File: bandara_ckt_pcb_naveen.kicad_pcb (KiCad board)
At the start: 2 copper layers, 98.8 x 78.6 mm, 54 parts, among them J1 Nanopore, U1 MCP4725xxx-xCH, U2 ADS1115IDGS, U3 AD820, U4 Dual Power Supply, U5 AD820, U6 AD820

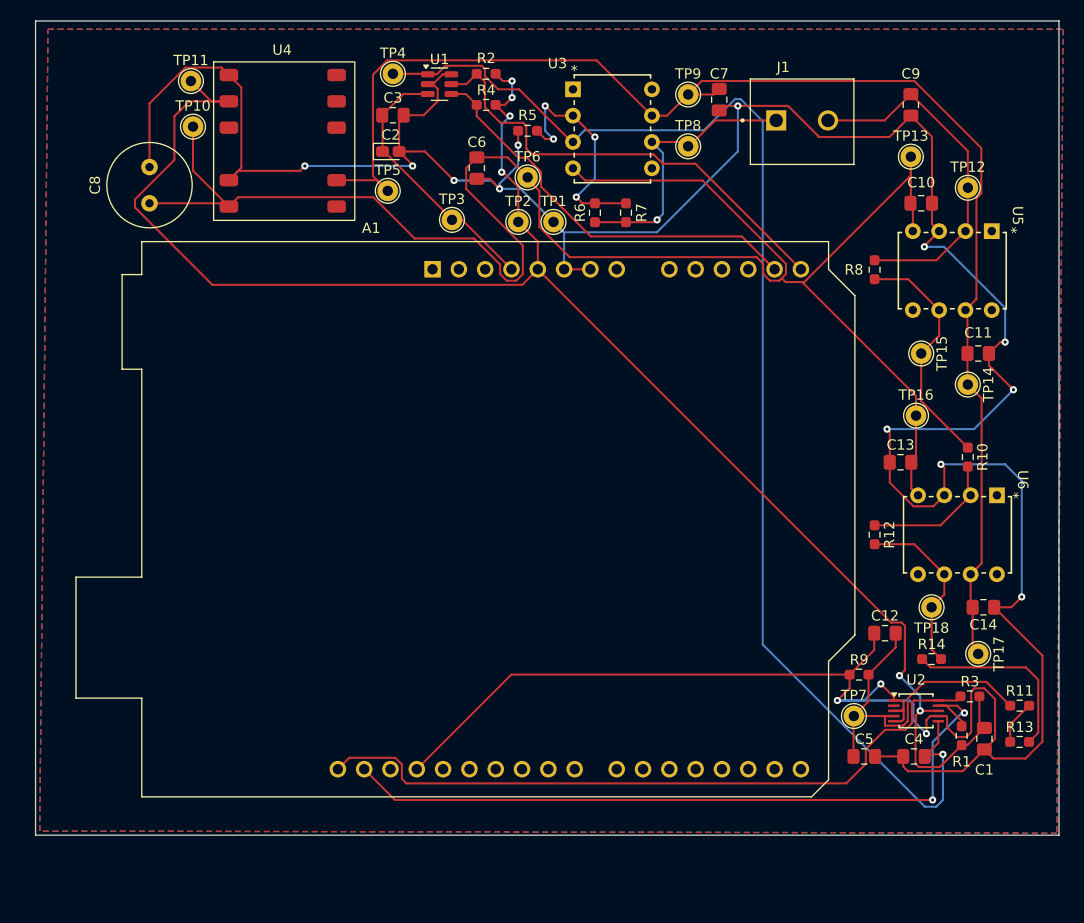
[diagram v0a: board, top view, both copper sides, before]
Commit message: Changes
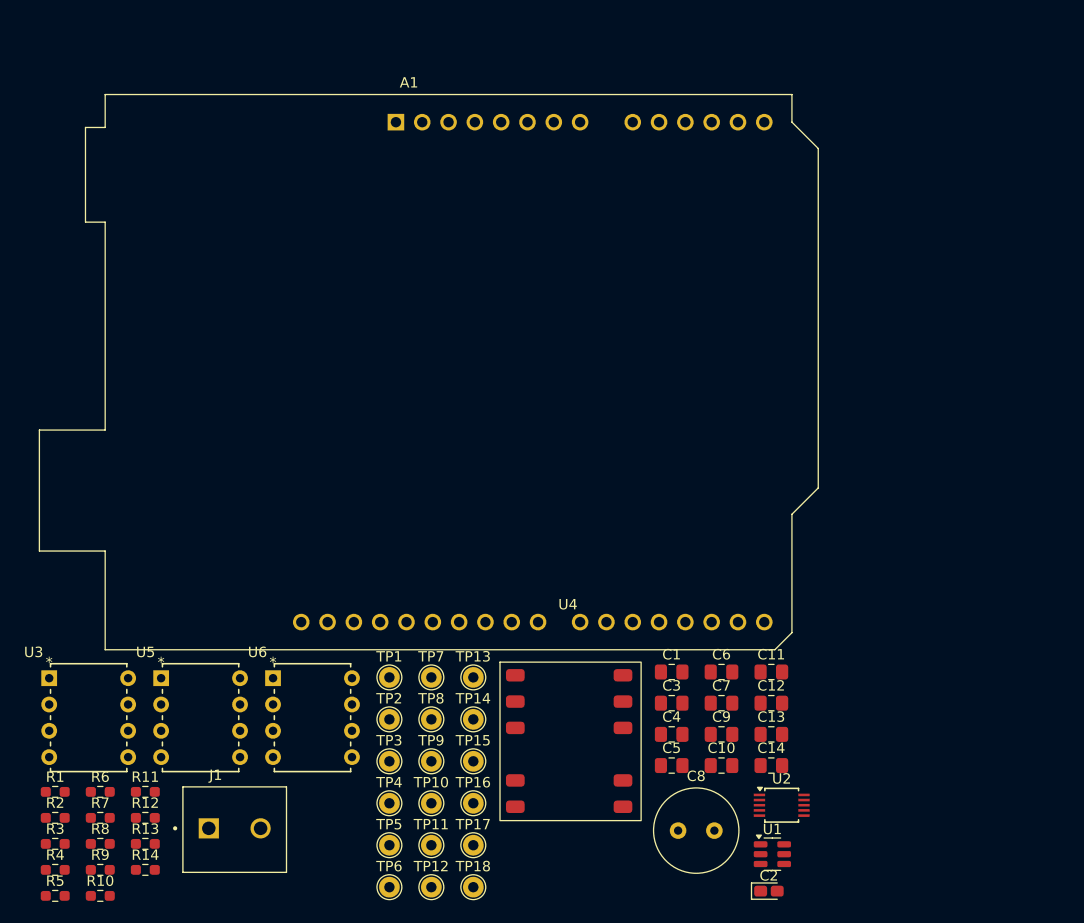
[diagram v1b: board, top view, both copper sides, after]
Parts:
- moved R10 93.9 mm to (46.2, 136.9), turned to 0 degrees
- moved R8 93.1 mm to (46.2, 131.8), turned to 0 degrees
- moved U5 91.1 mm to (52.1, 115.8), turned to 0 degrees
- moved R3 89.4 mm to (41.9, 131.8)
- moved R1 87.7 mm to (41.9, 126.8), turned to 0 degrees
- moved J1 87.6 mm to (54.2, 134.6)
- moved R5 86.8 mm to (41.9, 136.9), turned to 0 degrees
- moved TP12 85.1 mm to (78.2, 136.0)
- moved R13 85.0 mm to (50.6, 131.8)
- moved R11 84.8 mm to (50.6, 126.8)
- moved R4 84.8 mm to (41.9, 134.3), turned to 0 degrees
- moved R2 83.0 mm to (41.9, 129.3), turned to 0 degrees
- moved U1 81.0 mm to (111.1, 132.8)
- moved C2 80.2 mm to (110.8, 136.4)
- moved C8 79.2 mm to (102.0, 130.6), turned to 0 degrees
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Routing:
- net GND: track 355.5 -> 0.00 mm, vias 15 -> 0
- net -VSW: track 178.5 -> 0.00 mm
- net +5V: track 164.8 -> 0.00 mm, vias 6 -> 0
- net +VSW: track 136.8 -> 0.00 mm
- net Net-(U1-VOUT): track 127.0 -> 0.00 mm, vias 1 -> 0
- net Net-(U2-SDA): track 72.1 -> 0.00 mm, vias 2 -> 0
- net Net-(U2-SCL): track 67.9 -> 0.00 mm
- net Net-(U1-SCL): track 44.7 -> 0.00 mm
- net Net-(U1-SDA): track 39.7 -> 0.00 mm
- net Net-(U2-AIN0): track 35.2 -> 0.00 mm
- net Net-(J1-Pin_2): track 34.6 -> 0.00 mm
- net Net-(J1-Pin_1): track 27.5 -> 0.00 mm, vias 1 -> 0
- net +3.3V: track 26.0 -> 0.00 mm
- net Net-(U5-Vout): track 23.3 -> 0.00 mm
- net Net-(U3--IN): track 23.1 -> 0.00 mm, vias 4 -> 0
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- removed copper zone on B.Cu, net +5V
- removed copper zone on F.Cu, net +5V
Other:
- board outline removed
